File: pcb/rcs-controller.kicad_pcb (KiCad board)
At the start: 2 copper layers, 100 x 75 mm, 82 parts, among them J1 00222-32051, J10 0022-232021, J2 0022-232021, J3 0022-232041, J4 Screw_Terminal_4_P3.50mm, J8 00222-32051, Q1 SI7465DP-T1-E3, Q2 SI7465DP-T1-E3, Q3 SI7465DP-T1-E3, Q4 PMV45EN2, Q5 PMV45EN2, U1 LSM6DSOX, U2 MP26123DR-LF-Z, U3 TPS63070, U4 FeatherS3

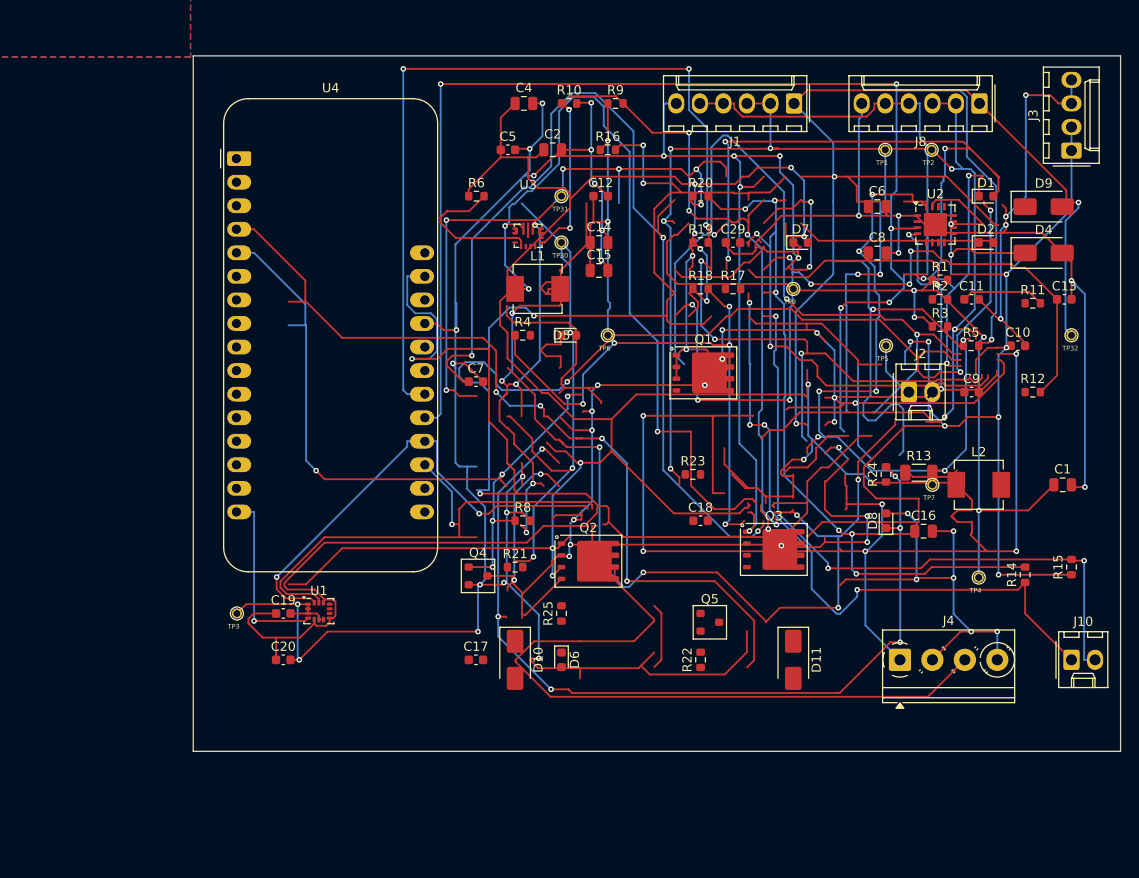
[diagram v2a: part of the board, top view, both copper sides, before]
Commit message: Rev2
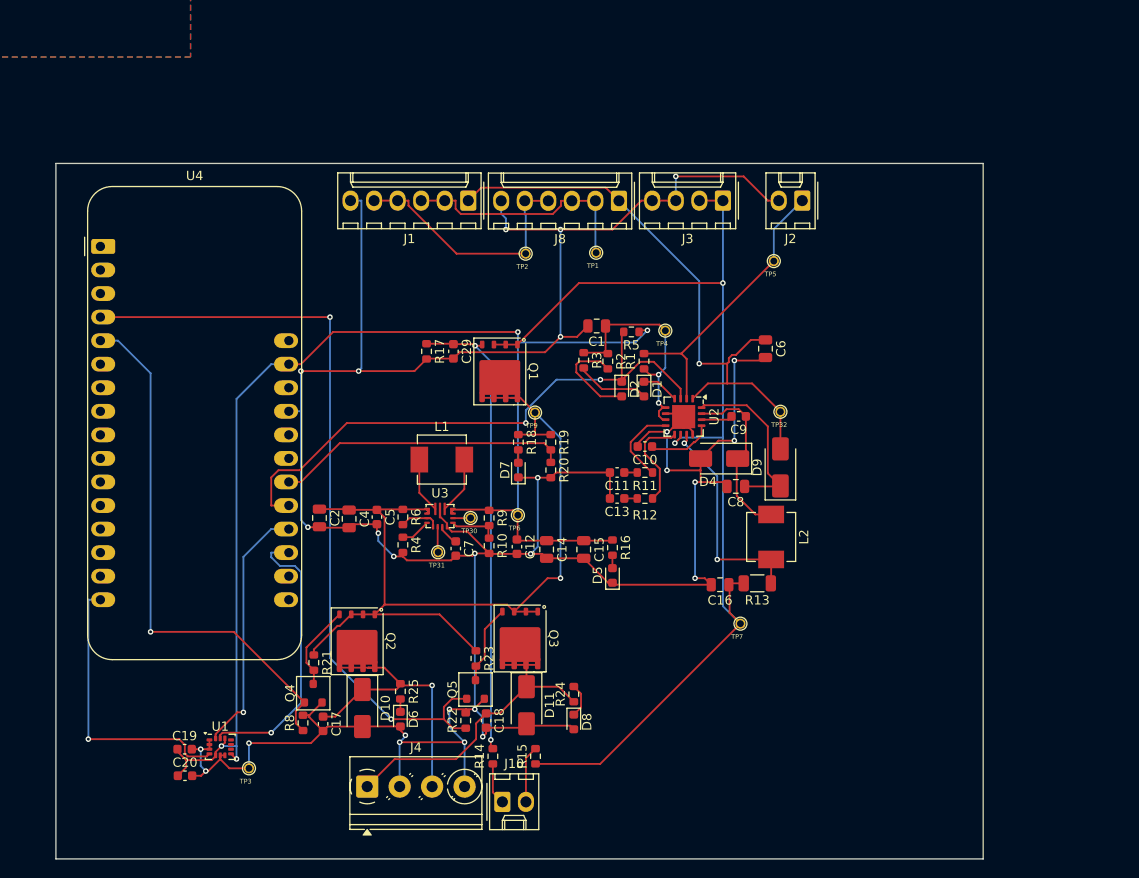
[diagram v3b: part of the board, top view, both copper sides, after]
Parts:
- moved J10 63.3 mm to (133.6, 145.3)
- moved R15 61.3 mm to (137.2, 140.4)
- moved R14 60.6 mm to (132.6, 140.4)
- moved J4 59.1 mm to (119.0, 143.7)
- moved C1 53.1 mm to (143.8, 94.0), turned to 180 degrees
- moved C13 52.8 mm to (146.0, 112.6), turned to 180 degrees
- moved C4 48.6 mm to (117.1, 114.8), turned to -90 degrees
- moved R10 48.5 mm to (132.2, 117.7), turned to -90 degrees
- moved C2 47.0 mm to (113.9, 114.7), turned to -90 degrees
- moved R9 46.7 mm to (132.2, 114.7), turned to -90 degrees
- moved R11 45.6 mm to (149.0, 109.8), turned to 180 degrees
- moved TP2 45.2 mm to (136.1, 86.2)
- moved R12 43.4 mm to (149.0, 112.6), turned to 180 degrees
- moved TP4 43.0 mm to (151.2, 94.5)
- moved R16 42.9 mm to (145.5, 117.9), turned to -90 degrees
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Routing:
- net GND: track 530.2 -> 349.0 mm, vias 42 -> 27
- net VBUS: track 285.0 -> 103.9 mm, vias 11 -> 1
- net +3.3V: track 306.5 -> 140.1 mm, vias 7 -> 4
- net CANH: track 177.3 -> 26.4 mm, vias 9 -> 0
- net Net-(Q2-G): track 159.9 -> 9.33 mm, vias 13 -> 0
- net +BATT: track 243.3 -> 117.7 mm, vias 16 -> 2
- net BATT_READ: track 145.2 -> 31.6 mm, vias 6 -> 0
- net Net-(D11-K): track 149.1 -> 37.5 mm, vias 6 -> 0
- net UMB_~{ON}: track 171.5 -> 63.1 mm, vias 6 -> 2
- net /Power/VUMB: track 170.8 -> 64.6 mm, vias 4 -> 1
- net Net-(U3-L2): track 111.3 -> 6.21 mm, vias 8 -> 0
- net Net-(U3-VAUX): track 105.7 -> 2.30 mm, vias 3 -> 0
- net Net-(D8-K): track 94.8 -> 3.68 mm, vias 6 -> 0
- net Net-(C13-Pad1): track 87.3 -> 1.40 mm, vias 7 -> 0
- net Net-(U3-L1): track 88.6 -> 6.04 mm, vias 3 -> 0
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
